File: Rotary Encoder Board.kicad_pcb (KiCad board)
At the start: 2 copper layers, 22.9 x 15 mm, 5 parts, among them J1 Conn_01x05, SW1 RotaryEncoder_Switch

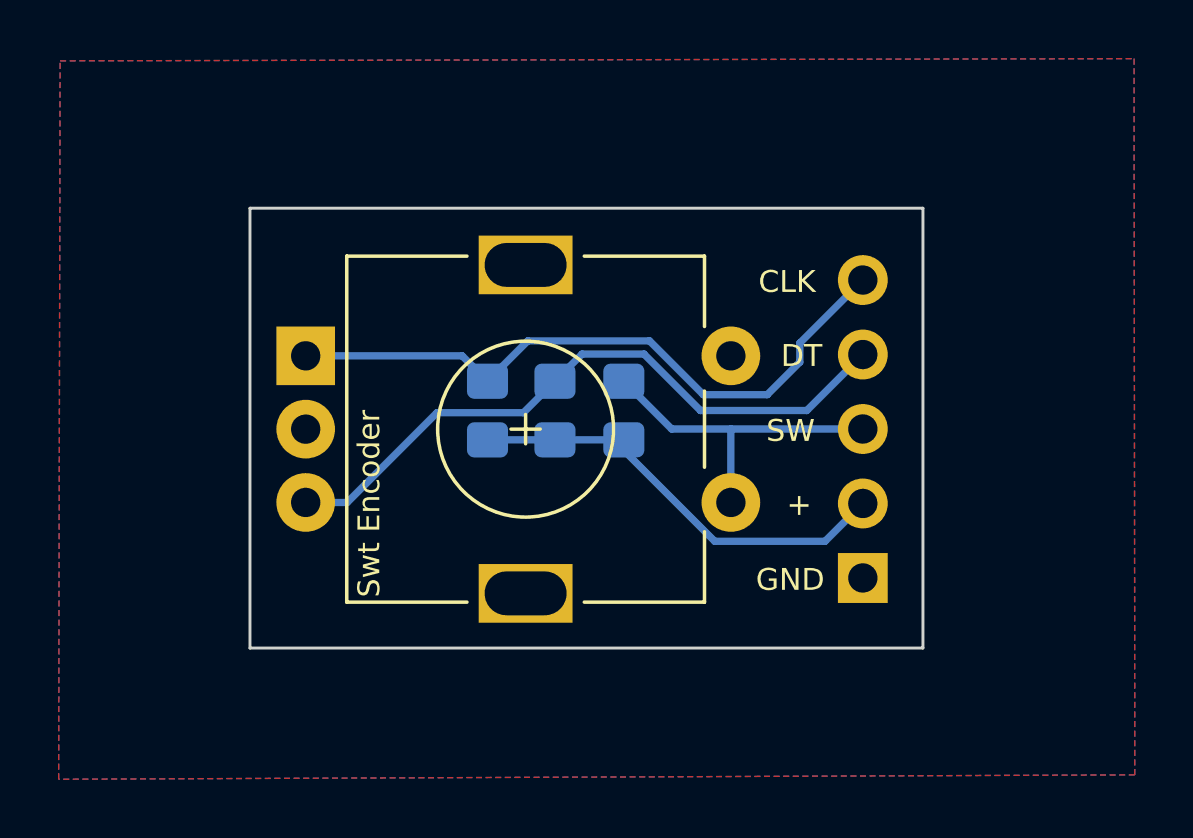
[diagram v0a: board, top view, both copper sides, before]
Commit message: sync everything
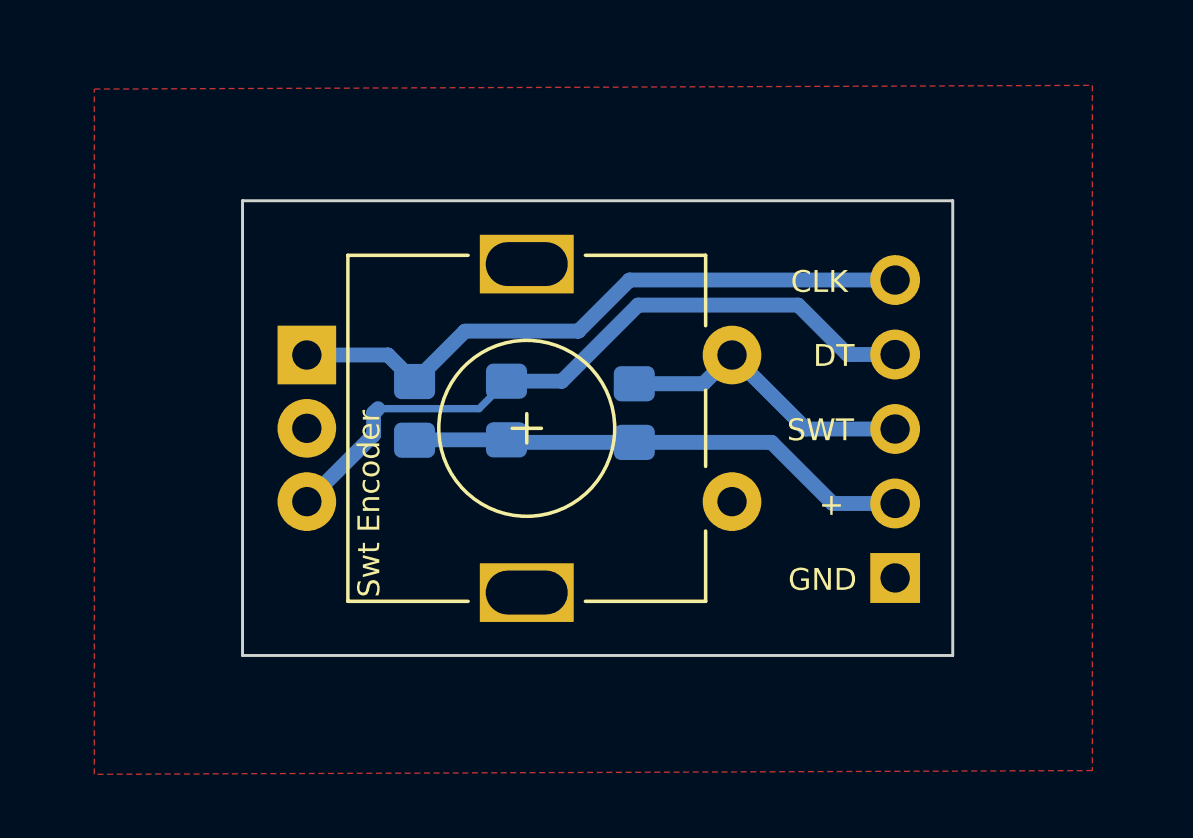
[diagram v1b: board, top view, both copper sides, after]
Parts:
- SW1: footprint Rotary_Encoder:RotaryEncoder_Alps_EC11E-Switch_Vertical_H20mm -> 000_Thomas_Footprints:Rotary Encoder
- moved SW1 8.04 mm to (139.7, 87.0)
- moved R2 2.49 mm to (135.8, 86.4)
- moved R1 1.65 mm to (138.9, 86.4)
- moved J1 1.10 mm to (152.2, 92.1)
- moved R3 0.37 mm to (143.3, 86.5)
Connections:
- SW1 pad S1: /SW -> GND
- SW1 pad S2: GND -> /SW
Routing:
- net +5V: track 15.0 -> 17.3 mm
- net /DT: track 22.7 -> 24.0 mm
- net /SW: track 11.3 -> 10.3 mm
- net /CLK: track 22.7 -> 21.9 mm
- removed copper zone on B.Cu, net GND
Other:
- board size 22.9 x 15 mm -> 24.2 x 15.5 mm
- board text added: "R3 pulls SWT high"
- board text added: "SWT"
- board text removed: "R3 pulls SW high"
- board text removed: "SW"
- board text removed: "https://github.com/Thomas1B"
